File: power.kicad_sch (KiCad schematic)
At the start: 26 parts, among them T1 WE-PPTI_1006, U14 MT3608

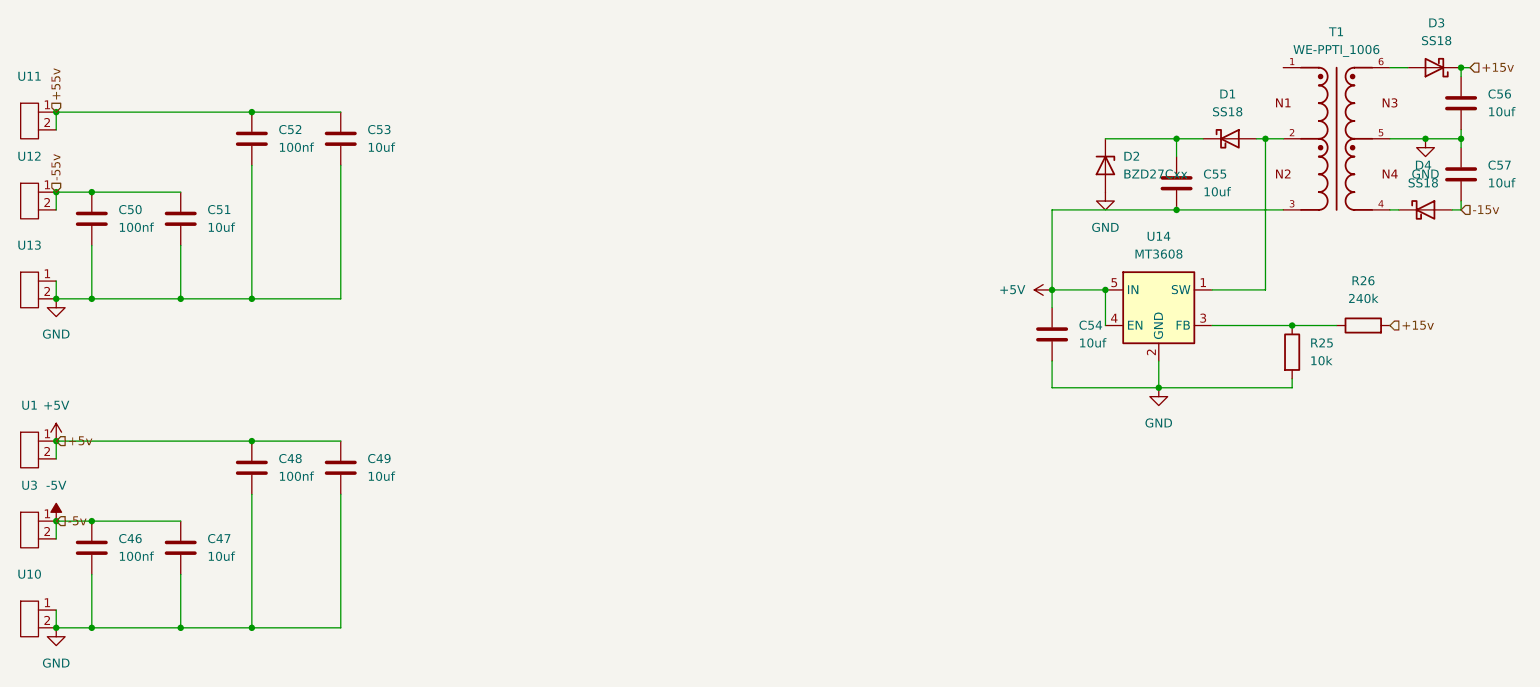
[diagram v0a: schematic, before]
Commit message: current routing stage
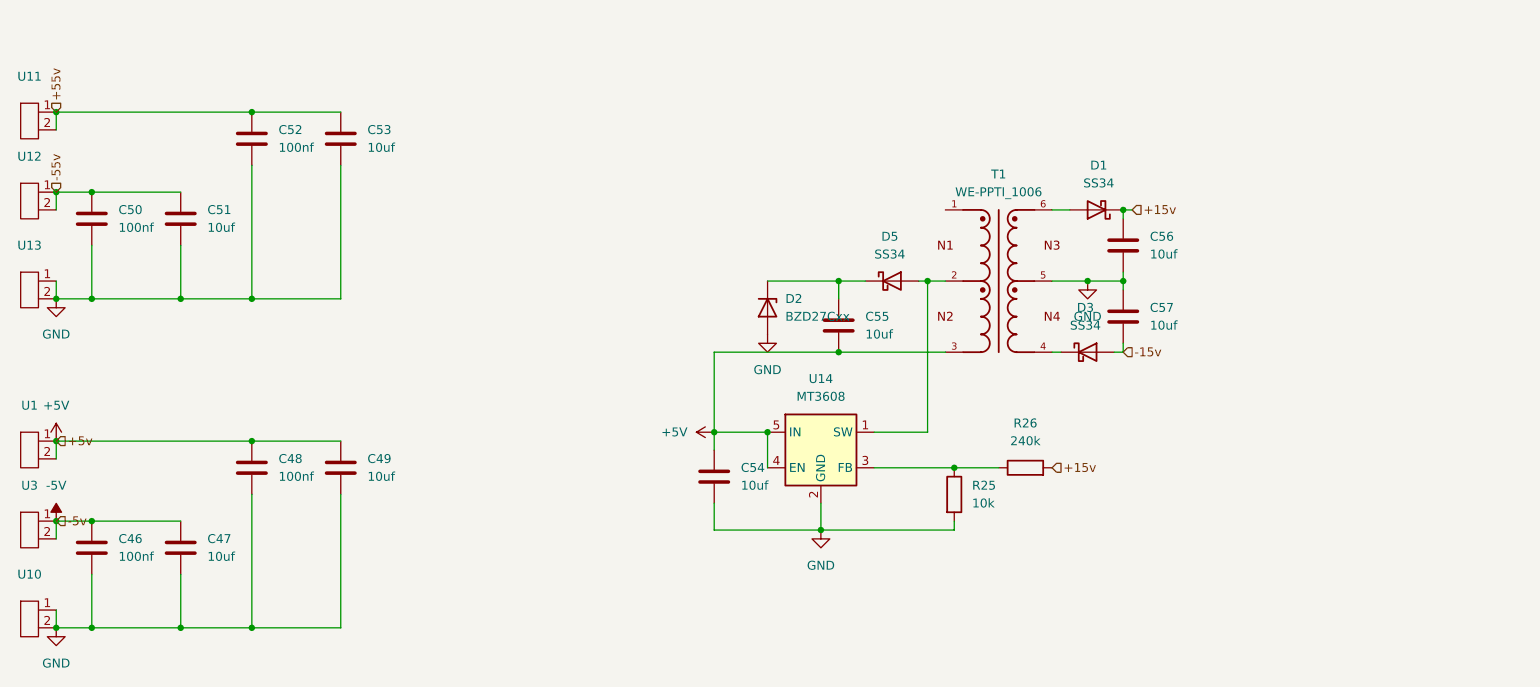
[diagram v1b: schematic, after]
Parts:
- removed D1, D3, D4: SS18, Diode_SMD:D_SMA, symbol Diode:SS18
- added D1, D3, D5: SS34, Diode_SMD:D_SMA, symbol Diode:SS34
- C46, C47, C48, C49, C50, C51, C52, C53, C54, C55, C56, C57, R25, R26: footprint (none) -> Capacitor_SMD:C_0805_2012Metric
- D2: footprint Diode_SMD:D_SMF -> Package_TO_SOT_SMD:SOT-23
- T1: footprint WE-PPTI_1006:WE-PPTI_1006_L10.2W6.73H4.19 -> WE-pptI_1006:WE-PPTI_1006_L10.2W6.73H4.19
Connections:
- net +15v: now also D1.1 (K)
- net -15v: now also D3.2 (A)
- net at T1.4: now also D3.1 (K)
- net at C55.1, D2.1 (K): now also D5.1 (K)
- net at T1.6: now also D1.2 (A)
- net at T1.2, U14.1 (SW): now also D5.2 (A)
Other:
- moved on the sheet: C54, C55, C56, C57, D2, R25, R26, T1, U14

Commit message: sim the new lpf
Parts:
- C46, C48, C50, C52, C54: footprint Capacitor_SMD:C_0805_2012Metric -> Capacitor_SMD:C_0201_0603Metric
- R25, R26: footprint Capacitor_SMD:C_0805_2012Metric -> Resistor_SMD:R_0201_0603Metric
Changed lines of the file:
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@@
 			)
 		)
-		(property "Footprint" "Capacitor_SMD:C_0805_2012Metric"
+		(property "Footprint" "Resistor_SMD:R_0201_0603Metric"
 			(at 174.752 88.9 90)
 			(effects
@@
 			)
 		)
-		(property "Footprint" "Capacitor_SMD:C_0805_2012Metric"
+		(property "Footprint" "Capacitor_SMD:C_0201_0603Metric"
 			(at 77.1652 41.91 0)
 			(effects
@@
 			)
 		)
-		(property "Footprint" "Capacitor_SMD:C_0805_2012Metric"
+		(property "Footprint" "Capacitor_SMD:C_0201_0603Metric"
 			(at 143.2052 90.17 0)
 			(effects
@@
 			)
 		)
-		(property "Footprint" "Capacitor_SMD:C_0805_2012Metric"
+		(property "Footprint" "Capacitor_SMD:C_0201_0603Metric"
 			(at 77.1652 88.9 0)
 			(effects
@@
 			)
 		)
-		(property "Footprint" "Capacitor_SMD:C_0805_2012Metric"
+		(property "Footprint" "Capacitor_SMD:C_0201_0603Metric"
 			(at 54.3052 53.34 0)
 			(effects
@@
 			)
 		)
-		(property "Footprint" "Capacitor_SMD:C_0805_2012Metric"
+		(property "Footprint" "Capacitor_SMD:C_0201_0603Metric"
 			(at 54.3052 100.33 0)
 			(effects
@@
 			)
 		)
-		(property "Footprint" "Capacitor_SMD:C_0805_2012Metric"
+		(property "Footprint" "Resistor_SMD:R_0201_0603Metric"
 			(at 186.69 86.868 90)
 			(effects

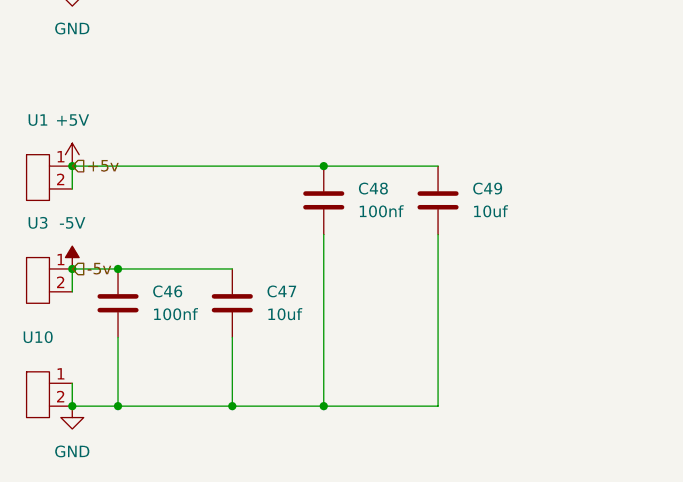
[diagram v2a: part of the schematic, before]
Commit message: routing draft 2
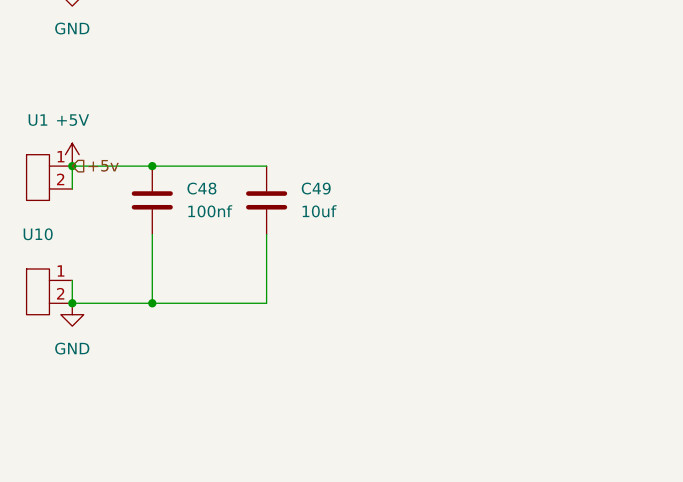
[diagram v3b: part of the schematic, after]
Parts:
- removed C46: 100nf, Capacitor_SMD:C_0201_0603Metric, symbol Device:C
- removed C47: 10uf, Capacitor_SMD:C_0805_2012Metric, symbol Device:C
- removed U3: ~, 1_Sockets:Untitled, symbol 1_variable gain:1_4mm_SOCKET
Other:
- moved on the sheet: C48, C49, U10
